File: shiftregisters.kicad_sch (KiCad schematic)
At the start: 10 parts, among them U1 74HC165, U2 74HC165, U3 74HC165, U4 74HC165, U5 74HC165

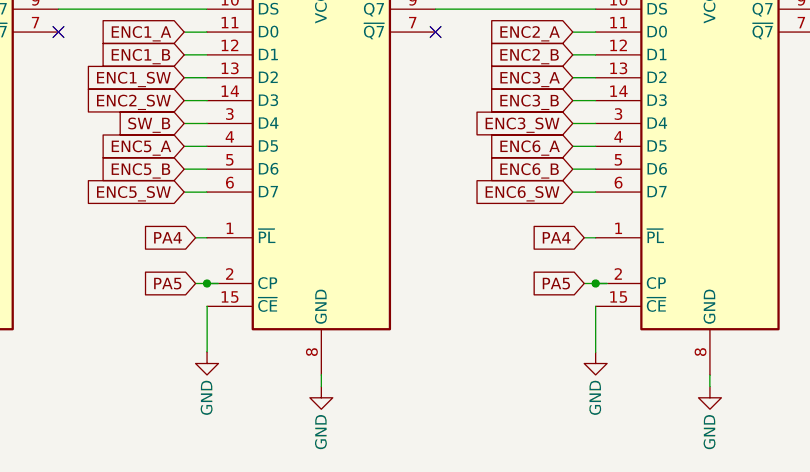
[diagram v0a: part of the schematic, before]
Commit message: Solve all warnings
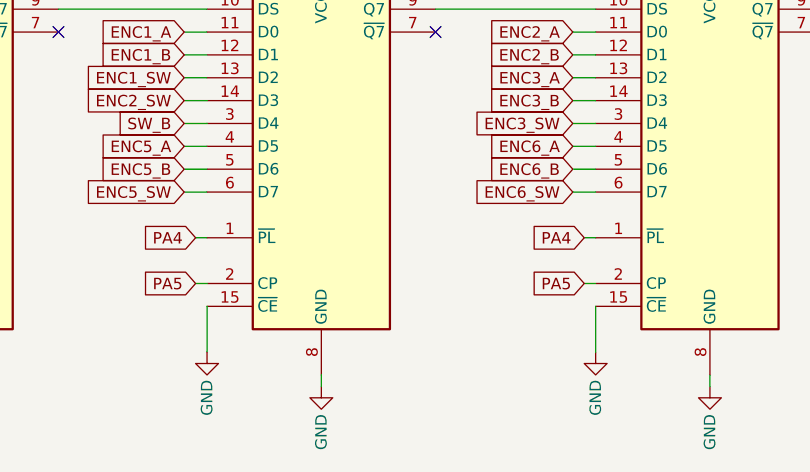
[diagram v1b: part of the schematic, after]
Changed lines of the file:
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@@
-	)
-	(junction
-		(at 130.81 80.01)
-		(diameter 0)
-		(color 0 0 0 0)
 	)
 	(junction
@@
 	)
 	(junction
-		(at 173.99 80.01)
-		(diameter 0)
-		(color 0 0 0 0)
-	)
-	(junction
 		(at 101.6 38.1)
 		(diameter 0)
@@
 	(wire
 		(pts
+			(xy 236.22 39.37) (xy 245.11 39.37)
+		)
+		(stroke
+			(width 0)
+			(type default)
+		)
+	)
+	(wire
+		(pts
+			(xy 215.9 54.61) (xy 218.44 54.61)
+		)
+		(stroke
+			(width 0)
+			(type default)
+		)
+	)
+	(wire
+		(pts
+			(xy 171.45 62.23) (xy 173.99 62.23)
+		)
+		(stroke
+			(width 0)
+			(type default)
+		)
+	)
+	(wire
+		(pts
+			(xy 143.51 35.56) (xy 143.51 38.1)
+		)
+		(stroke
+			(width 0)
+			(type default)
+		)
+	)
+	(wire
+		(pts
+			(xy 128.27 69.85) (xy 130.81 69.85)
+		)
+		(stroke
+			(width 0)
+			(type default)
+		)
+	)
+	(wire
+		(pts
+			(xy 101.6 38.1) (xy 101.6 41.91)
+		)
+		(stroke
+			(width 0)
+			(type default)
+		)
+	)
+	(wire
+		(pts
+			(xy 186.69 35.56) (xy 186.69 38.1)
+		)
+		(stroke
+			(width 0)
+			(type default)
+		)
+	)
+	(wire
+		(pts
+			(xy 171.45 54.61) (xy 173.99 54.61)
+		)
+		(stroke
+			(width 0)
+			(type default)
+		)
+	)
+	(wire
+		(pts
+			(xy 218.44 82.55) (xy 218.44 87.63)
+		)
+		(stroke
+			(width 0)
+			(type default)
+		)
+	)
+	(wire
+		(pts
+			(xy 128.27 54.61) (xy 130.81 54.61)
+		)
+		(stroke
+			(width 0)
+			(type default)
+		)
+	)
+	(wire
+		(pts
+			(xy 46.99 82.55) (xy 46.99 87.63)
+		)
+		(stroke
+			(width 0)
+			(type default)
+		)
+	)
+	(wire
+		(pts
+			(xy 87.63 80.01) (xy 88.9 80.01)
+		)
+		(stroke
+			(width 0)
+			(type default)
+		)
+	)
+	(wire
+		(pts
+			(xy 186.69 90.17) (xy 186.69 91.44)
+		)
+		(stroke
+			(width 0)
+			(type default)
+		)
+	)
+	(wire
+		(pts
 			(xy 172.72 80.01) (xy 173.99 80.01)
 		)
@@
 	(wire
 		(pts
-			(xy 236.22 39.37) (xy 245.11 39.37)
-		)
-		(stroke
-			(width 0)
-			(type default)
-		)
-	)
-	(wire
-		(pts
-			(xy 215.9 54.61) (xy 218.44 54.61)
-		)
-		(stroke
-			(width 0)
-			(type default)
-		)
-	)
-	(wire
-		(pts
-			(xy 171.45 62.23) (xy 173.99 62.23)
-		)
-		(stroke
-			(width 0)
-			(type default)
-		)
-	)
-	(wire
-		(pts
-			(xy 143.51 35.56) (xy 143.51 38.1)
-		)
-		(stroke
-			(width 0)
-			(type default)
-		)
-	)
-	(wire
-		(pts
-			(xy 128.27 69.85) (xy 130.81 69.85)
-		)
-		(stroke
-			(width 0)
-			(type default)
-		)
-	)
-	(wire
-		(pts
-			(xy 101.6 38.1) (xy 101.6 41.91)
-		)
-		(stroke
-			(width 0)
-			(type default)
-		)
-	)
-	(wire
-		(pts
-			(xy 186.69 35.56) (xy 186.69 38.1)
-		)
-		(stroke
-			(width 0)
-			(type default)
-		)
-	)
-	(wire
-		(pts
-			(xy 171.45 54.61) (xy 173.99 54.61)
-		)
-		(stroke
-			(width 0)
-			(type default)
-		)
-	)
-	(wire
-		(pts
-			(xy 218.44 82.55) (xy 218.44 87.63)
-		)
-		(stroke
-			(width 0)
-			(type default)
-		)
-	)
-	(wire
-		(pts
-			(xy 128.27 54.61) (xy 130.81 54.61)
-		)
-		(stroke
-			(width 0)
-			(type default)
-		)
-	)
-	(wire
-		(pts
-			(xy 46.99 82.55) (xy 46.99 87.63)
-		)
-		(stroke
-			(width 0)
-			(type default)
-		)
-	)
-	(wire
-		(pts
-			(xy 87.63 80.01) (xy 88.9 80.01)
-		)
-		(stroke
-			(width 0)
-			(type default)
-		)
-	)
-	(wire
-		(pts
-			(xy 186.69 90.17) (xy 186.69 91.44)
-		)
-		(stroke
-			(width 0)
-			(type default)
-		)
-	)
-	(wire
-		(pts
 			(xy 171.45 57.15) (xy 173.99 57.15)
 		)
@@
 	(wire
 		(pts
+			(xy 129.54 80.01) (xy 130.81 80.01)
+		)
+		(stroke
+			(width 0)
+			(type default)
+		)
+	)
+	(wire
+		(pts
 			(xy 148.59 38.1) (xy 157.48 38.1)
 		)
@@
 	(wire
 		(pts
-			(xy 129.54 80.01) (xy 130.81 80.01)
-		)
-		(stroke
-			(width 0)
-			(type default)
-		)
-	)
-	(wire
-		(pts
 			(xy 215.9 57.15) (xy 218.44 57.15)
 		)
@@
 	(wire
 		(pts
-			(xy 130.81 80.01) (xy 132.08 80.01)
-		)
-		(stroke
-			(width 0)
-			(type default)
-		)
-	)
-	(wire
-		(pts
 			(xy 44.45 54.61) (xy 46.99 54.61)
 		)
@@
 		)
 		(stroke
-			(width 0)
-			(type default)
-		)
-	)
-	(wire
-		(pts
-			(xy 173.99 80.01) (xy 175.26 80.01)
-		)
-		(stroke

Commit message: Added jack symbols and footprints also footprints for ics and caps
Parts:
- C29, C30, C31, C32, C33: footprint (none) -> Capacitor_SMD:C_0603_1608Metric
- U1, U2, U3, U4, U5: footprint (none) -> diggi_footprints:SOP65P640X120-16
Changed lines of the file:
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@@
 			)
 		)
-		(property "Footprint" ""
+		(property "Footprint" "diggi_footprints:SOP65P640X120-16"
 			(at 101.6 64.77 0)
 			(effects
@@
 			)
 		)
-		(property "Footprint" ""
+		(property "Footprint" "Capacitor_SMD:C_0603_1608Metric"
 			(at 62.23 38.1 0)
 			(effects
@@
 			)
 		)
-		(property "Footprint" ""
+		(property "Footprint" "diggi_footprints:SOP65P640X120-16"
 			(at 59.69 64.77 0)
 			(effects
@@
 			)
 		)
-		(property "Footprint" ""
+		(property "Footprint" "Capacitor_SMD:C_0603_1608Metric"
 			(at 233.68 39.37 0)
 			(effects
@@
 			)
 		)
-		(property "Footprint" ""
+		(property "Footprint" "Capacitor_SMD:C_0603_1608Metric"
 			(at 146.05 38.1 0)
 			(effects
@@
 			)
 		)
-		(property "Footprint" ""
+		(property "Footprint" "Capacitor_SMD:C_0603_1608Metric"
 			(at 104.14 38.1 0)
 			(effects
@@
 			)
 		)
-		(property "Footprint" ""
+		(property "Footprint" "diggi_footprints:SOP65P640X120-16"
 			(at 231.14 64.77 0)
 			(effects
@@
 			)
 		)
-		(property "Footprint" ""
+		(property "Footprint" "diggi_footprints:SOP65P640X120-16"
 			(at 186.69 64.77 0)
 			(effects
@@
 			)
 		)
-		(property "Footprint" ""
+		(property "Footprint" "diggi_footprints:SOP65P640X120-16"
 			(at 143.51 64.77 0)
 			(effects
@@
 			)
 		)
-		(property "Footprint" ""
+		(property "Footprint" "Capacitor_SMD:C_0603_1608Metric"
 			(at 189.23 38.1 0)
 			(effects
